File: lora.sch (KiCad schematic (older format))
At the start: 1 part, among them U1 SX1301

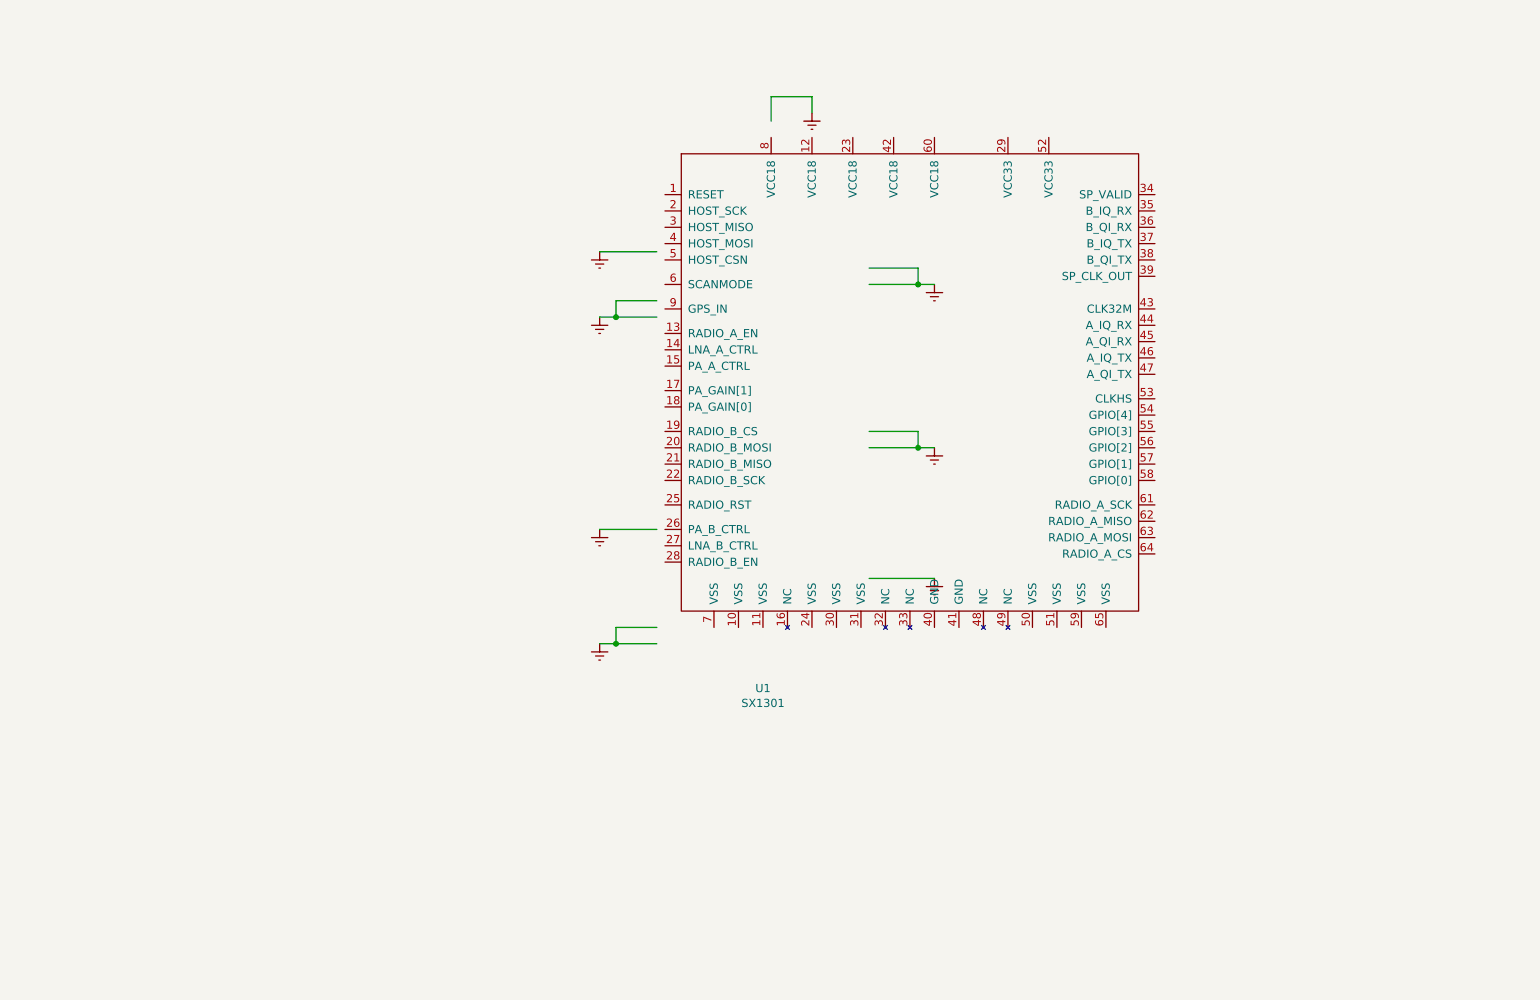
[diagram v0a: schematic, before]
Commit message: partialy wired - sequential pins
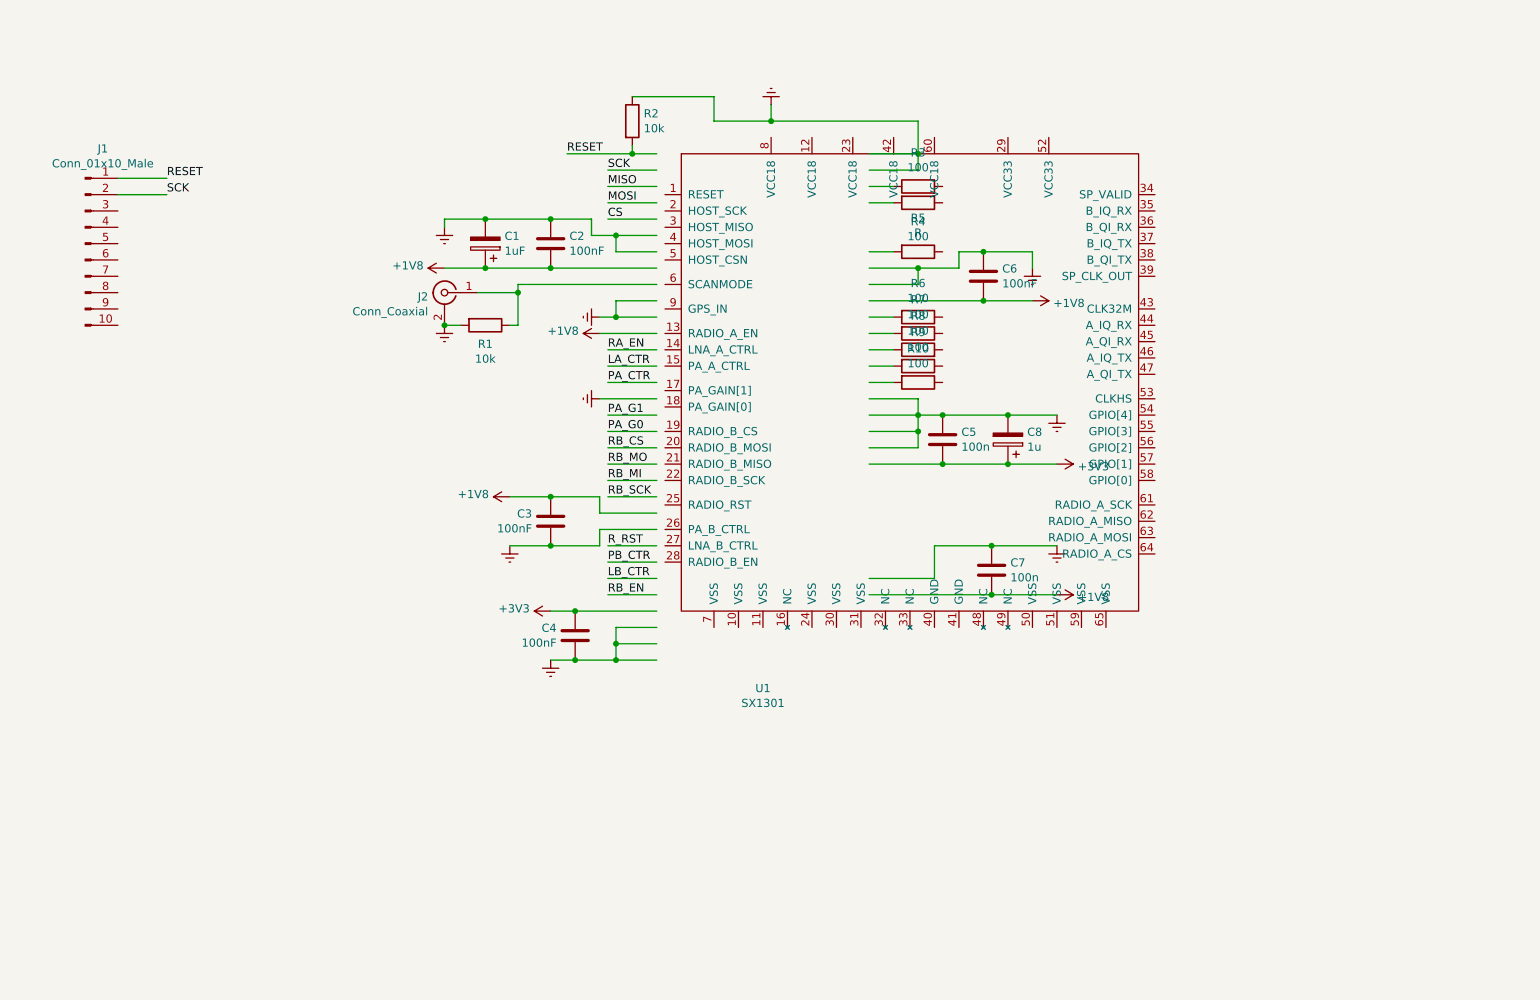
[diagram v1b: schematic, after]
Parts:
- added C1: 1uF, symbol Device:CP
- added C2, C3, C4, C6: 100nF, Capacitor_SMD:C_0603_1608Metric_Pad1.05x0.95mm_HandSolder, symbol Device:C
- added C5, C7: 100n, Capacitor_SMD:C_0603_1608Metric_Pad1.05x0.95mm_HandSolder, symbol Device:C
- added C8: 1u, symbol Device:CP
- added J1: Conn_01x10_Male, Connector_PinHeader_2.54mm:PinHeader_1x10_P2.54mm_Vertical, symbol Connector:Conn_01x10_Male
- added J2: Conn_Coaxial, symbol Connector:Conn_Coaxial
- added R1, R2: 10k, Resistor_SMD:R_0603_1608Metric_Pad1.05x0.95mm_HandSolder, symbol Device:R
- added R10, R3, R4, R6, R7, R8, R9: 100, Resistor_SMD:R_0603_1608Metric_Pad1.05x0.95mm_HandSolder, symbol Device:R
- added R5: R, Resistor_SMD:R_0603_1608Metric_Pad1.05x0.95mm_HandSolder, symbol Device:R
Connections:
- net labels added: +1V8, +3V3, CS, LA_CTR, LB_CTR, MISO, MOSI, PA_CTR, PA_G0, PA_G1, PB_CTR, RA_EN, RB_CS, RB_EN, RB_MI, RB_MO, RB_SCK, RESET, R_RST, SCK
- wire segments 22 -> 109

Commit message: v1.0
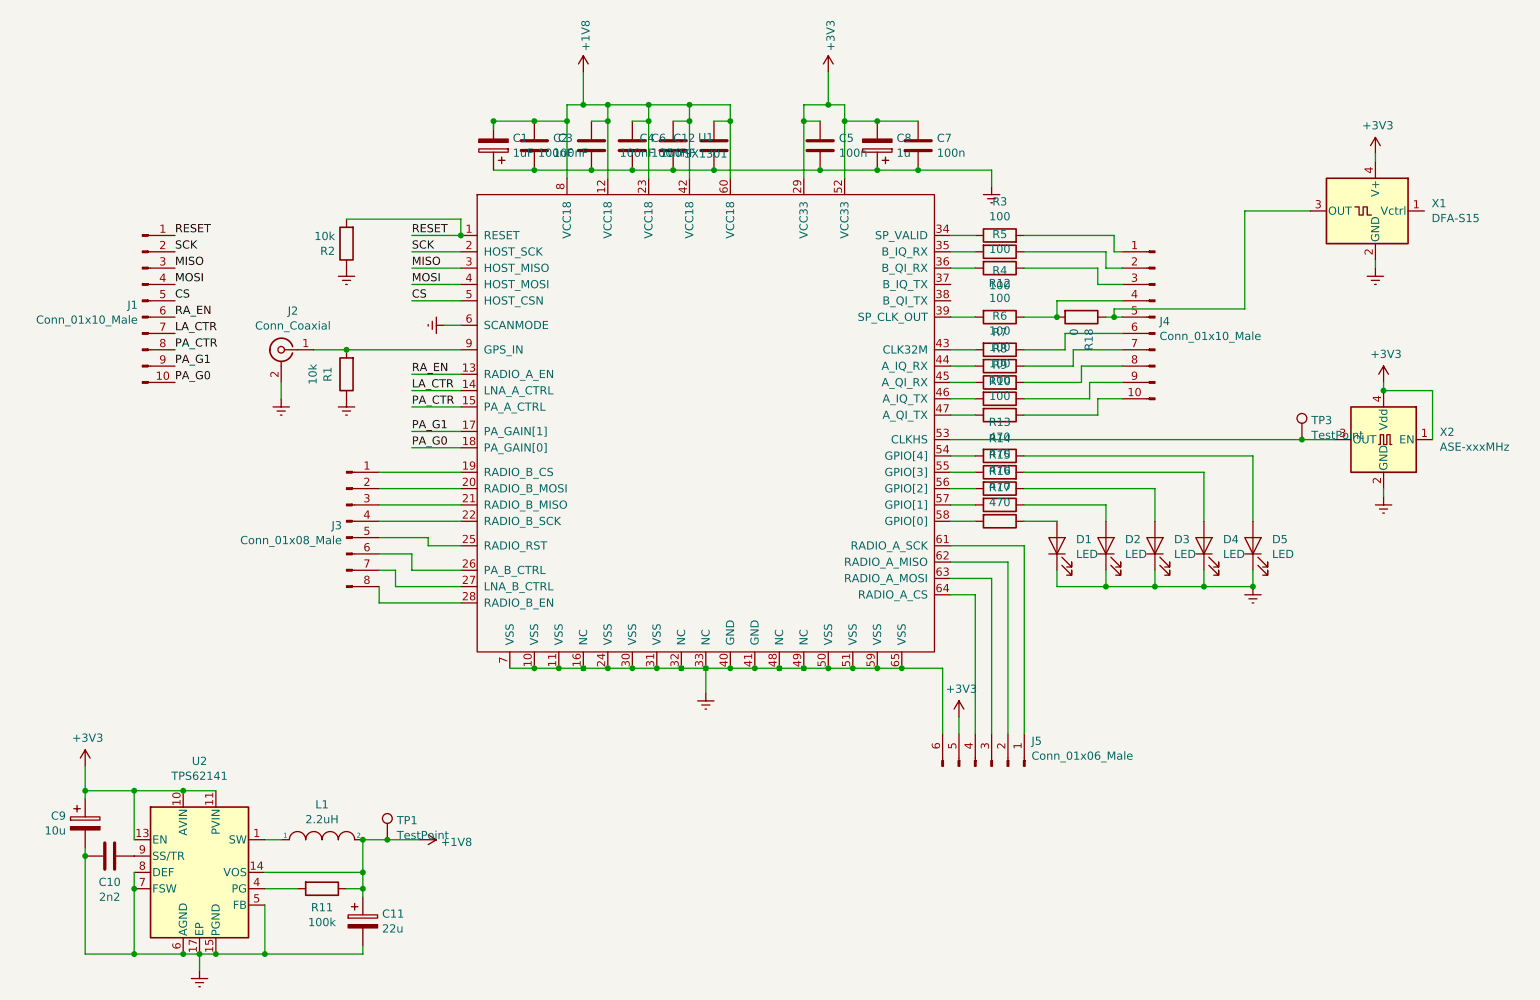
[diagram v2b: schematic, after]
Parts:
- added C10: 2n2, Capacitor_SMD:C_0402_1005Metric, symbol Device:C
- added C11: 22u, Capacitor_SMD:C_0603_1608Metric, symbol Device:CP
- added C12: 100nF, Capacitor_SMD:C_0402_1005Metric, symbol Device:C
- added C9: 10u, Capacitor_SMD:C_0603_1608Metric, symbol Device:CP
- added D1, D2, D3, D4, D5: LED, LED_SMD:LED_0402_1005Metric, symbol Device:LED
- added J3: Conn_01x08_Male, Connector_PinHeader_2.54mm:PinHeader_1x08_P2.54mm_Vertical, symbol Connector:Conn_01x08_Male
- added J4: Conn_01x10_Male, Connector_PinHeader_2.54mm:PinHeader_1x10_P2.54mm_Vertical, symbol Connector:Conn_01x10_Male
- added J5: Conn_01x06_Male, Connector_PinHeader_2.54mm:PinHeader_1x06_P2.54mm_Vertical, symbol Connector:Conn_01x06_Male
- added L1: 2.2uH, Inductor_SMD:L_6.3x6.3_H3, symbol pspice:INDUCTOR
- added R11: 100k, Resistor_SMD:R_0402_1005Metric, symbol Device:R
- added R12: 100, Resistor_SMD:R_0402_1005Metric, symbol Device:R
- added R13, R14, R15, R16, R17: 470, Resistor_SMD:R_0402_1005Metric, symbol Device:R
- added R18: 0, Resistor_SMD:R_0402_1005Metric, symbol Device:R
- added TP1, TP3: TestPoint, TestPoint:TestPoint_THTPad_1.5x1.5mm_Drill0.7mm, symbol Connector:TestPoint
- added U2: TPS62141, Package_DFN_QFN:QFN-16-1EP_3x3mm_P0.5mm_EP1.8x1.8mm, symbol Regulator_Switching:TPS62141
- added X1: DFA-S15, Oscillator:Oscillator_SMD_Fordahl_DFAS15-4Pin_5.0x3.2mm, symbol Oscillator:DFA-S15
- added X2: ASE-xxxMHz, Oscillator:Oscillator_SMD_Abracon_ASE-4Pin_3.2x2.5mm, symbol Oscillator:ASE-xxxMHz
- C1, C8: footprint (none) -> Capacitor_SMD:C_0603_1608Metric
- C2, C3, C4, C5, C6, C7: footprint Capacitor_SMD:C_0603_1608Metric_Pad1.05x0.95mm_HandSolder -> Capacitor_SMD:C_0402_1005Metric
- J2: footprint (none) -> Connector_Coaxial:U.FL_Molex_MCRF_73412-0110_Vertical
- R1, R10, R2, R3, R4, R6, R7, R8, R9: footprint Resistor_SMD:R_0603_1608Metric_Pad1.05x0.95mm_HandSolder -> Resistor_SMD:R_0402_1005Metric
- R5: value R -> 100; footprint Resistor_SMD:R_0603_1608Metric_Pad1.05x0.95mm_HandSolder -> Resistor_SMD:R_0402_1005Metric
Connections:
- net labels removed: LB_CTR, PB_CTR, RB_CS, RB_EN, RB_MI, RB_MO, RB_SCK, R_RST
- wire segments 109 -> 203
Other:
- moved on the sheet: C1, C2, C3, C4, C5, C6, C7, C8, J2, R1, R10, R2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
